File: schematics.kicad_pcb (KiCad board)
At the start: 2 copper layers, 13 parts, among them J1 Conn_01x12_Pin, SW1 SW_Push, SW10 SW_Push, SW11 SW_Push, SW12 SW_Push, SW2 SW_Push, SW3 SW_Push, SW4 SW_Push, SW5 SW_Push, SW6 SW_Push, SW7 SW_Push, SW8 SW_Push, SW9 SW_Push

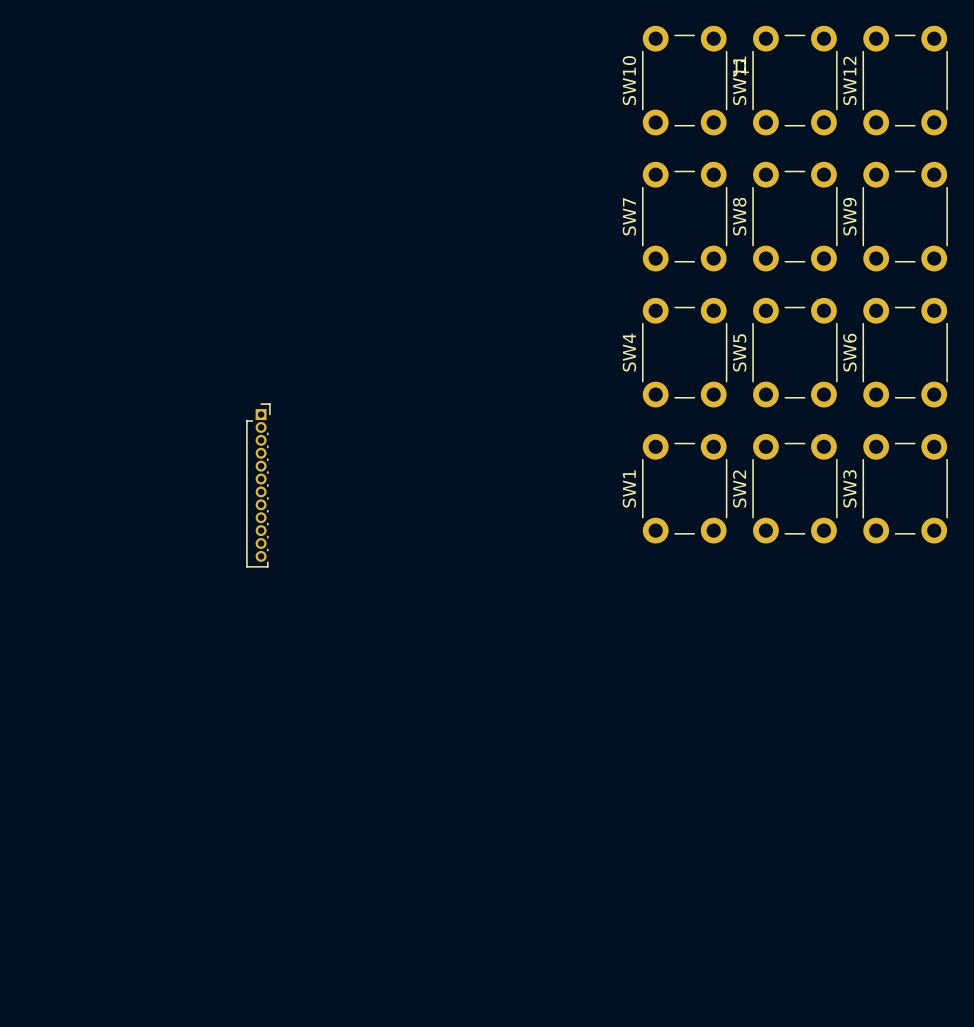
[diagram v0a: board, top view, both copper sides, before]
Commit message: initial commit
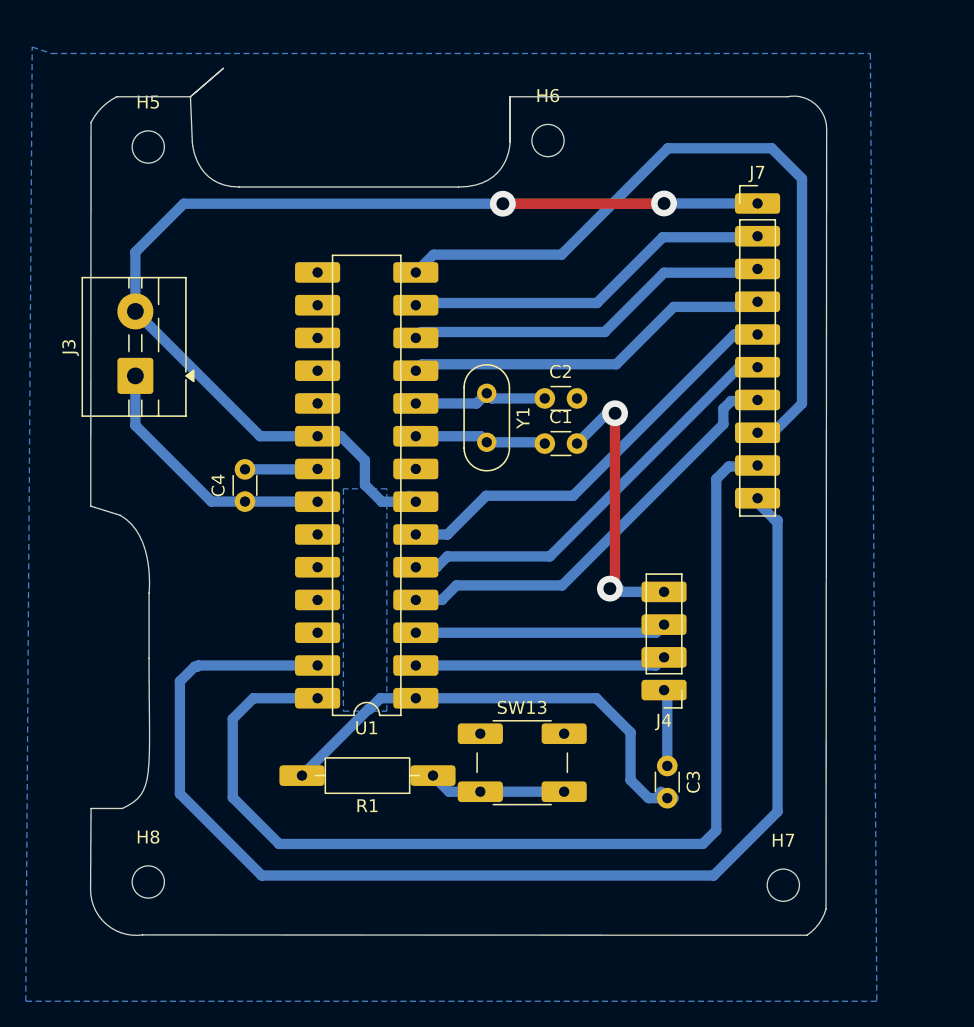
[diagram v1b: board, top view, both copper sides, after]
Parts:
- removed J1: Conn_01x12_Pin, Connector_PinSocket_1.00mm:PinSocket_1x12_P1.00mm_Vertical
- removed SW1, SW10, SW11, SW12, SW2, SW3, SW4, SW5, SW6, SW7, SW8, SW9: SW_Push, Button_Switch_THT:SW_PUSH_6mm
- added C1: C, Capacitor_THT:C_Disc_D3.0mm_W1.6mm_P2.50mm, F.Cu at (107.2, 75.2)
- added C2: C, Capacitor_THT:C_Disc_D3.0mm_W1.6mm_P2.50mm, F.Cu at (107.2, 71.8)
- added C3: C, Capacitor_THT:C_Disc_D3.0mm_W1.6mm_P2.50mm, F.Cu at (116.8, 100.2)
- added C4: C, Capacitor_THT:C_Disc_D3.0mm_W1.6mm_P2.50mm, F.Cu at (84.0, 79.8)
- added H5: MountingHole, MountingHole:MountingHole_2.5mm, F.Cu at (76.5, 52.2)
- added H6: MountingHole, MountingHole:MountingHole_2.5mm, F.Cu at (107.5, 51.8)
- added H7: MountingHole, MountingHole:MountingHole_2.5mm, F.Cu at (125.8, 109.5)
- added H8: MountingHole, MountingHole:MountingHole_2.5mm, F.Cu at (76.5, 109.2)
- added J3: Screw_Terminal_01x02, TerminalBlock:TerminalBlock_MaiXu_MX126-5.0-02P_1x02_P5.00mm, F.Cu at (75.5, 70.0)
- added J4: Conn_01x04_Pin, Connector_PinHeader_2.54mm:PinHeader_1x04_P2.54mm_Vertical, F.Cu at (116.5, 94.4)
- added J7: Conn_01x10_Pin, Connector_PinHeader_2.54mm:PinHeader_1x10_P2.54mm_Vertical, F.Cu at (123.8, 56.6)
- added R1: 10k, Resistor_THT:R_Axial_DIN0207_L6.3mm_D2.5mm_P10.16mm_Horizontal, F.Cu at (98.6, 101.0)
- added SW13: SW_Push, Button_Switch_THT:SW_PUSH_6mm, F.Cu at (102.2, 97.8)
- added U1: ATmega328P-P, Package_DIP:DIP-28_W7.62mm, F.Cu at (97.2, 95.0)
- added Y1: Crystal, Crystal:Crystal_HC52-6mm_Vertical, F.Cu at (102.8, 71.3)
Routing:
- net Net-(J7-Pin_10): track 0.00 -> 96.1 mm
- net +5V: track 0.00 -> 85.0 mm, vias 0 -> 2
- net Net-(J7-Pin_9): track 0.00 -> 83.4 mm
- net Net-(J7-Pin_8): track 0.00 -> 57.0 mm
- net GND: track 0.00 -> 42.0 mm, vias 0 -> 2
- net Net-(U1-~{RESET}/PC6): track 0.00 -> 37.4 mm
- net Net-(J7-Pin_7): track 0.00 -> 33.3 mm
- net Net-(J7-Pin_5): track 0.00 -> 32.7 mm
- net Net-(J7-Pin_6): track 0.00 -> 32.6 mm
- net Net-(J7-Pin_3): track 0.00 -> 28.4 mm
- net Net-(J7-Pin_4): track 0.00 -> 28.4 mm
- net Net-(J7-Pin_2): track 0.00 -> 28.4 mm
- net Net-(J4-Pin_3): track 0.00 -> 19.5 mm
- net Net-(J4-Pin_2): track 0.00 -> 19.5 mm
- net Net-(R1-Pad1): track 0.00 -> 10.7 mm
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- added copper zone on B.Cu, net GND
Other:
- board outline added: 57.1 x 67.3 mm
